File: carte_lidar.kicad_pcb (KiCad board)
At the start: 2 copper layers, 68 x 68 mm, 26 parts, among them J1 Conn_01x03_Pin, J2 Conn_01x02_Pin, J3 Conn_01x05_Socket, J4 Conn_01x02, J5 Conn_01x04_Socket, U1 TPS54302, U2 Pico

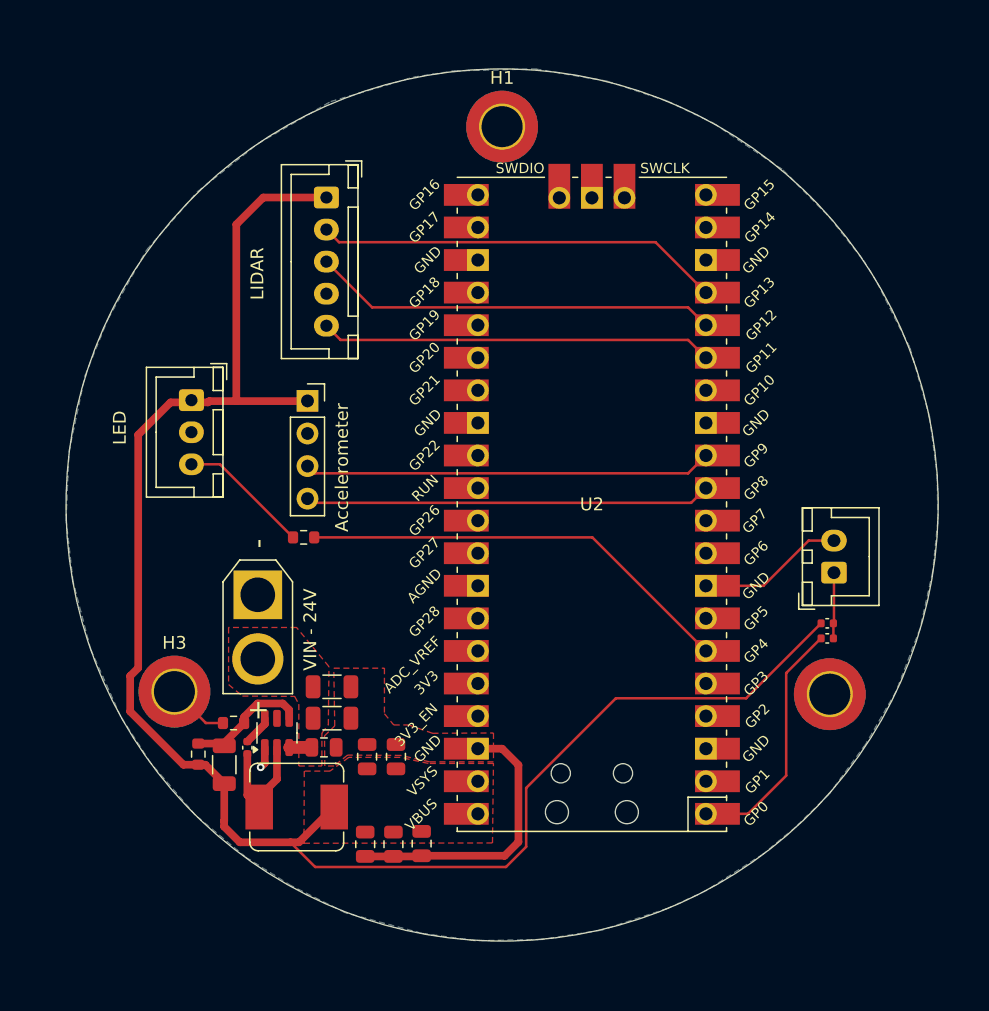
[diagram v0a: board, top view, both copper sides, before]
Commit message: update all
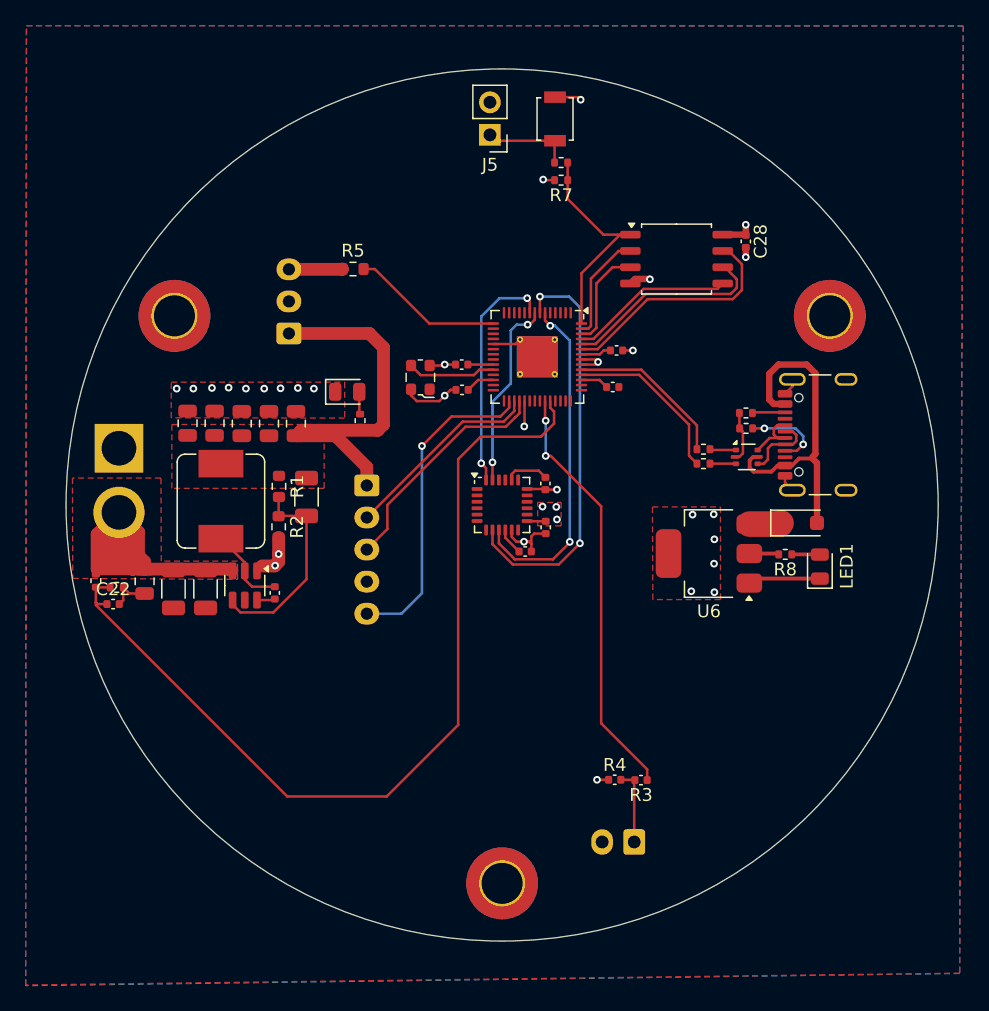
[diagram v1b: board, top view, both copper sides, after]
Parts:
- added C21: 0.1uF 10V, Capacitor_SMD:C_0402_1005Metric, F.Cu at (101.8, 103.6)
- added C22: 220nF 50V, Capacitor_SMD:C_0402_1005Metric, F.Cu at (69.7, 107.7)
- added C23: 2.2nF 10V, Capacitor_SMD:C_0402_1005Metric, F.Cu at (103.4, 98.3)
- added C24: 0.1uF 10V, Capacitor_SMD:C_0402_1005Metric, F.Cu at (103.4, 101.8)
- added C25: 0.1uF 10V, Capacitor_SMD:C_0402_1005Metric, F.Cu at (108.9, 88.0)
- added C26: 1uF 10V, Capacitor_SMD:C_0402_1005Metric, F.Cu at (108.6, 90.8)
- added C27: 0.1uF 10V, Capacitor_SMD:C_0402_1005Metric, F.Cu at (96.8, 89.0)
- added C28: 220nF 16V, Capacitor_SMD:C_0402_1005Metric, F.Cu at (119.0, 79.4)
- added D1: MBR120VLSFT1G, Diode_SMD:D_SOD-123F, F.Cu at (123.2, 101.4)
- added J6: USB_C_Receptacle_USB2.0, Connector_USB:USB_C_Receptacle_GCT_USB4105-xx-A_16P_TopMnt_Horizontal, F.Cu at (125.7, 94.5)
- added LED1: YELLOW, LED_SMD:LED_0805_2012Metric, F.Cu at (124.8, 104.8)
- added LED2: YELLOW, LED_SMD:LED_0805_2012Metric, F.Cu at (87.9, 91.2)
- added R11: 5.1k, Resistor_SMD:R_0402_1005Metric, F.Cu at (119.0, 94.0)
- added R12: 5.1k, Resistor_SMD:R_0402_1005Metric, F.Cu at (119.0, 92.8)
- added R13: 27R, Resistor_SMD:R_0402_1005Metric, F.Cu at (115.7, 96.8)
- added R14: 27R, Resistor_SMD:R_0402_1005Metric, F.Cu at (115.7, 95.7)
- added R15: 1k, Resistor_SMD:R_0402_1005Metric, F.Cu at (88.9, 93.4)
- added R16: 10k, Capacitor_SMD:C_0402_1005Metric, F.Cu at (96.9, 91.0)
- added R17: 5.1k, Resistor_SMD:R_0402_1005Metric, F.Cu at (68.3, 105.9)
- added R18: 1k, Resistor_SMD:R_0402_1005Metric, F.Cu at (70.0, 106.4)
- added R6: 1k, Resistor_SMD:R_0402_1005Metric, F.Cu at (104.6, 73.3)
- added R7: 100k, Resistor_SMD:R_0402_1005Metric, F.Cu at (104.6, 74.7)
- added R8: 1k, Resistor_SMD:R_0402_1005Metric, F.Cu at (122.1, 103.8)
- added SW1: SW_Push, Button_Switch_SMD:SW_SPST_B3U-1000P, F.Cu at (104.1, 69.9)
- added U3: W25Q128JVS, Package_SO:SOIC-8_5.23x5.23mm_P1.27mm, F.Cu at (113.6, 80.8)
- added U5: USBLC6-2P6, Package_TO_SOT_SMD:SOT-666, F.Cu at (119.1, 96.2)
- added U6: NM/AMS1117-3.3, Package_TO_SOT_SMD:SOT-223-3_TabPin2, F.Cu at (116.1, 103.8)
- added U7: MPU-6000, Sensor_Motion:InvenSense_QFN-24_4x4mm_P0.5mm, F.Cu at (100.0, 100.0)
- added X1: S2D12.000000B20F30T, Oscillator:Oscillator_SMD_ECS_2520MV-xxx-xx-4Pin_2.5x2.0mm, F.Cu at (93.6, 90.0)
- J1, J2, J3, J4: moved to B.Cu
- J5: value Conn_01x04_Socket -> Conn_01x02_Pin; footprint Connector_PinSocket_2.54mm:PinSocket_1x04_P2.54mm_Vertical -> Connector_PinHeader_2.54mm:PinHeader_1x02_P2.54mm_Vertical
- U2: value Pico -> RP2040; footprint MCU_RaspberryPi_and_Boards:RPi_Pico_SMD_TH -> Package_DFN_QFN:QFN-56-1EP_7x7mm_P0.4mm_EP3.2x3.2mm_ThermalVias
- moved H2 59.0 mm to (74.5, 85.2)
- moved C6 35.7 mm to (77.6, 93.6), turned to 90 degrees
- moved C8 34.8 mm to (81.8, 93.7), turned to 90 degrees
- moved C7 34.2 mm to (79.7, 93.7), turned to 90 degrees
- moved H3 29.6 mm to (100.0, 129.5)
- moved C10 29.5 mm to (75.5, 93.6)
- moved H1 29.5 mm to (125.5, 85.2)
- moved J4 27.9 mm to (109.0, 126.3), turned to 180 degrees
- moved C9 27.1 mm to (83.9, 93.7)
- moved J5 25.2 mm to (99.0, 71.1), turned to 180 degrees
- moved L1 24.6 mm to (78.1, 99.7), turned to 90 degrees
- moved J3 22.7 mm to (89.5, 98.5)
- moved C5 21.8 mm to (84.8, 99.4), turned to -90 degrees
- moved R1 21.8 mm to (82.6, 98.5), turned to -90 degrees
- moved R5 21.3 mm to (88.4, 81.6)
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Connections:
- net 24V renamed /power/VBAT
- C10 pad 1: 5V -> +5V
- C5 pad 1: 5V -> +5V
- C6 pad 1: 5V -> +5V
- C7 pad 1: 5V -> +5V
- C8 pad 1: 5V -> +5V
- C9 pad 1: 5V -> +5V
- J1 pad 1: 5V -> +5V
- J1 pad 3: /led -> Net-(J1-Pin_3)
- J3 pad 1: 5V -> +5V
- J5 pad 1: 5V -> Net-(J5-Pin_1)
- L1 pad 2: 5V -> +5V
- R1 pad 1: 5V -> +5V
- R3 pad 1: AU -> /AU
- R4 pad 1: 5V -> +3V3
- R5 pad 1: /led -> Net-(J1-Pin_3)
- R5 pad 2: Net-(U2-GPIO4) -> /led
- U2 pad 1: AU -> +3V3
- U2 pad 10: unconnected-(U2-GPIO7-Pad10) -> +3V3
- U2 pad 11: /sda -> unconnected-(U2-GPIO8-Pad11)
- U2 pad 12: /scl -> unconnected-(U2-GPIO9-Pad12)
- U2 pad 13: GND -> unconnected-(U2-GPIO10-Pad13)
- U2 pad 15: /motoct -> /led
- U2 pad 16: /lidar_rx -> unconnected-(U2-GPIO13-Pad16)
- U2 pad 17: /lidar_tx -> unconnected-(U2-GPIO14-Pad17)
- U2 pad 18: GND -> unconnected-(U2-GPIO15-Pad18)
- U2 pad 19: unconnected-(U2-GPIO14-Pad19) -> GND
- U2 pad 22: unconnected-(U2-GPIO17-Pad22) -> +3V3
- U2 pad 23: GND -> /+1.1V
- U2 pad 24: unconnected-(U2-GPIO18-Pad24) -> /Clk_12MHz
- U2 pad 26: unconnected-(U2-GPIO20-Pad26) -> Net-(U2-RUN)
- U2 pad 28: GND -> unconnected-(U2-GPIO17-Pad28)
- U2 pad 3: GND -> unconnected-(U2-GPIO1-Pad3)
- U2 pad 30: unconnected-(U2-RUN-Pad30) -> /motoct
- U2 pad 31: unconnected-(U2-GPIO26_ADC0-Pad31) -> /lidar_tx
- U2 pad 32: unconnected-(U2-GPIO27_ADC1-Pad32) -> /lidar_rx
- U2 pad 33: unconnected-(U2-AGND-Pad33) -> +3V3
- U2 pad 37: unconnected-(U2-3V3_EN-Pad37) -> /AU
- U2 pad 38: GND -> BAT_SENSE
- U2 pad 39: 5V -> unconnected-(U2-GPIO27_ADC1-Pad39)
- U2 pad 40: 5V -> unconnected-(U2-GPIO28_ADC2-Pad40)
- U2 pad 42: GND -> +3V3
- U2 pad 43: unconnected-(U2-SWDIO-Pad43) -> +3V3
- U2 pad 6: Net-(U2-GPIO4) -> /MISO
- U2 pad 7: unconnected-(U2-GPIO5-Pad7) -> /CSn
- U2 pad 8: GND -> /SCLK
- U2 pad 9: unconnected-(U2-GPIO6-Pad9) -> /MOSI
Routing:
- net 5V: track 133.8 -> 0.00 mm
- net BAT_SENSE: track 0.00 -> 71.4 mm
- net +5V: track 0.00 -> 34.3 mm
- net Net-(U2-GPIO4): track 34.2 -> 0.00 mm
- net /AU: track 0.00 -> 33.1 mm, vias 0 -> 2
- net /CSn: track 0.00 -> 32.4 mm, vias 0 -> 2
- net /scl: track 31.9 -> 0.00 mm
- net /sda: track 31.7 -> 0.00 mm
- net /MISO: track 0.00 -> 26.6 mm, vias 0 -> 2
- net Net-(D1-A): track 0.00 -> 26.3 mm
- net /power/VBAT: track 1.72 -> 27.3 mm
- net AU: track 19.3 -> 0.00 mm
- net Net-(U2-QSPI_SD3): track 0.00 -> 18.4 mm
- net /MOSI: track 0.00 -> 18.3 mm, vias 0 -> 2
- net Net-(U2-QSPI_SS): track 0.00 -> 17.9 mm
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- added copper zone on F.Cu, net +3V3
- added copper zone on In2.Cu, net +3V3
- added copper zone on F.Cu, net +5V
- added copper zone on In1.Cu, net GND
- removed copper zone on F.Cu, net 5V
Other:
- copper layers 2 -> 4
- board text added: "Opossum carte lidar 2025"
- board text removed: "Accelerometer"
- board text removed: "LED"
- board text removed: "LIDAR"
- board text removed: "VIN - 24V"
